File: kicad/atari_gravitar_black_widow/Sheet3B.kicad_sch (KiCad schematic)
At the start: 106 parts, among them Q1 2N3904, Y1 12.096 MHZ

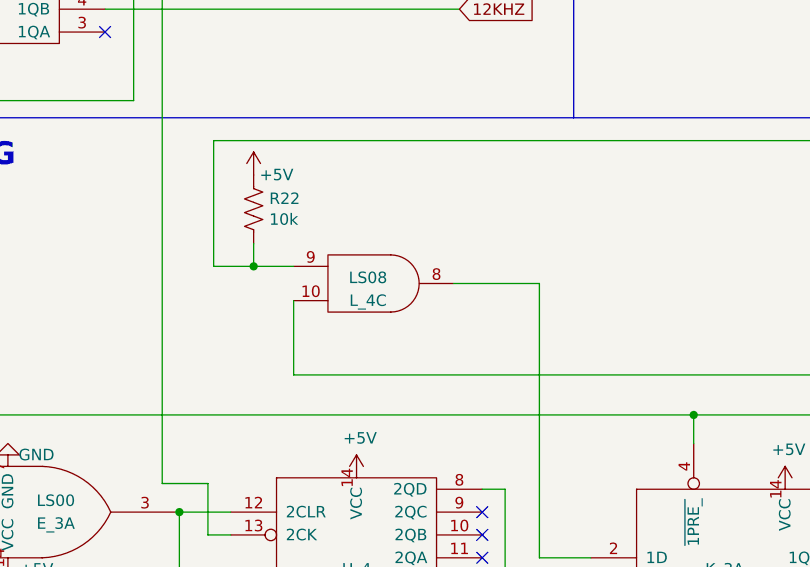
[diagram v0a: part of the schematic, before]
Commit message: 4A DONE
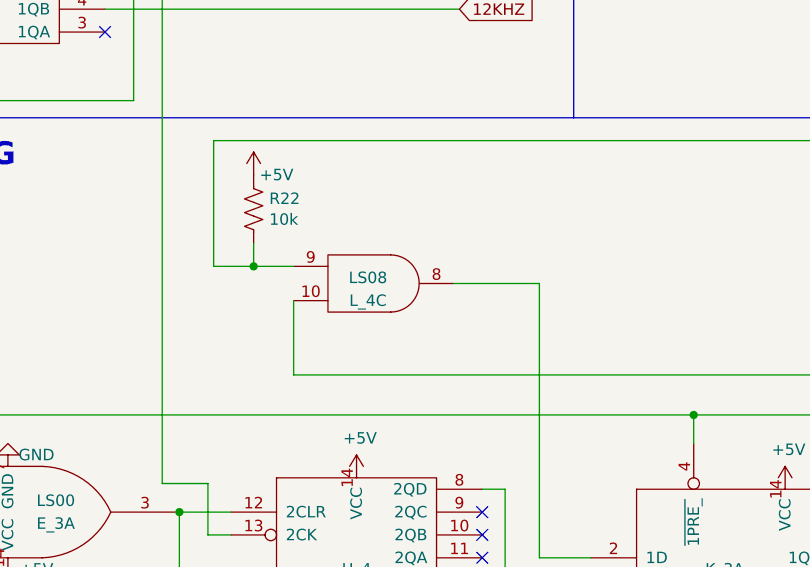
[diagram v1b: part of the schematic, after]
